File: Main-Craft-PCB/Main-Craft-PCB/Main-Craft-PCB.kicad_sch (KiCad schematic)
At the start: 216 parts, among them J1 Conn_01x10, J1 UART_1, J10 S500_2, J11 S500_3, J12 S500_4, J13 SOL_1, J14 SOL_2, J15 RELAY_1, J16 RELAY_2, J17 RELAY_3, J18 RELAY_3, J19 SOL_3, J2 UART_2, J20 SOL_4, J21 PWR_IN, J23 BAT_IN, J24 VESC_1, J25 VESC_2, J26 VESC_3, J27 VESC_4, J3 UART_3, J4 UART_4, J5 LEDS, J6 LEDS, J7 LEDS, J8 LEDS, J9 S500_1, Q1 TIP120, Q10 S9013, Q11 S9013, Q12 S9013, Q13 S9013, Q14 S9013, Q16 S9013, Q2 TIP120, Q25 IRFR9014PBF, Q3 TIP120, Q4 TIP120, Q5 S9013, Q6 S9013, Q7 S9013, Q8 S9013, Q9 S9013, U10 BFU590GX, U10 ZLDO1117G50TA, U2 NUCLEO144-F429ZI, U2 Pi Pico, U3 ESP8266, U4 LM358DR2G, U4 SN74LV4052, U5 74HC14, U5 LM358DR2G, U8 74HC14, U9 ZSR330GTA

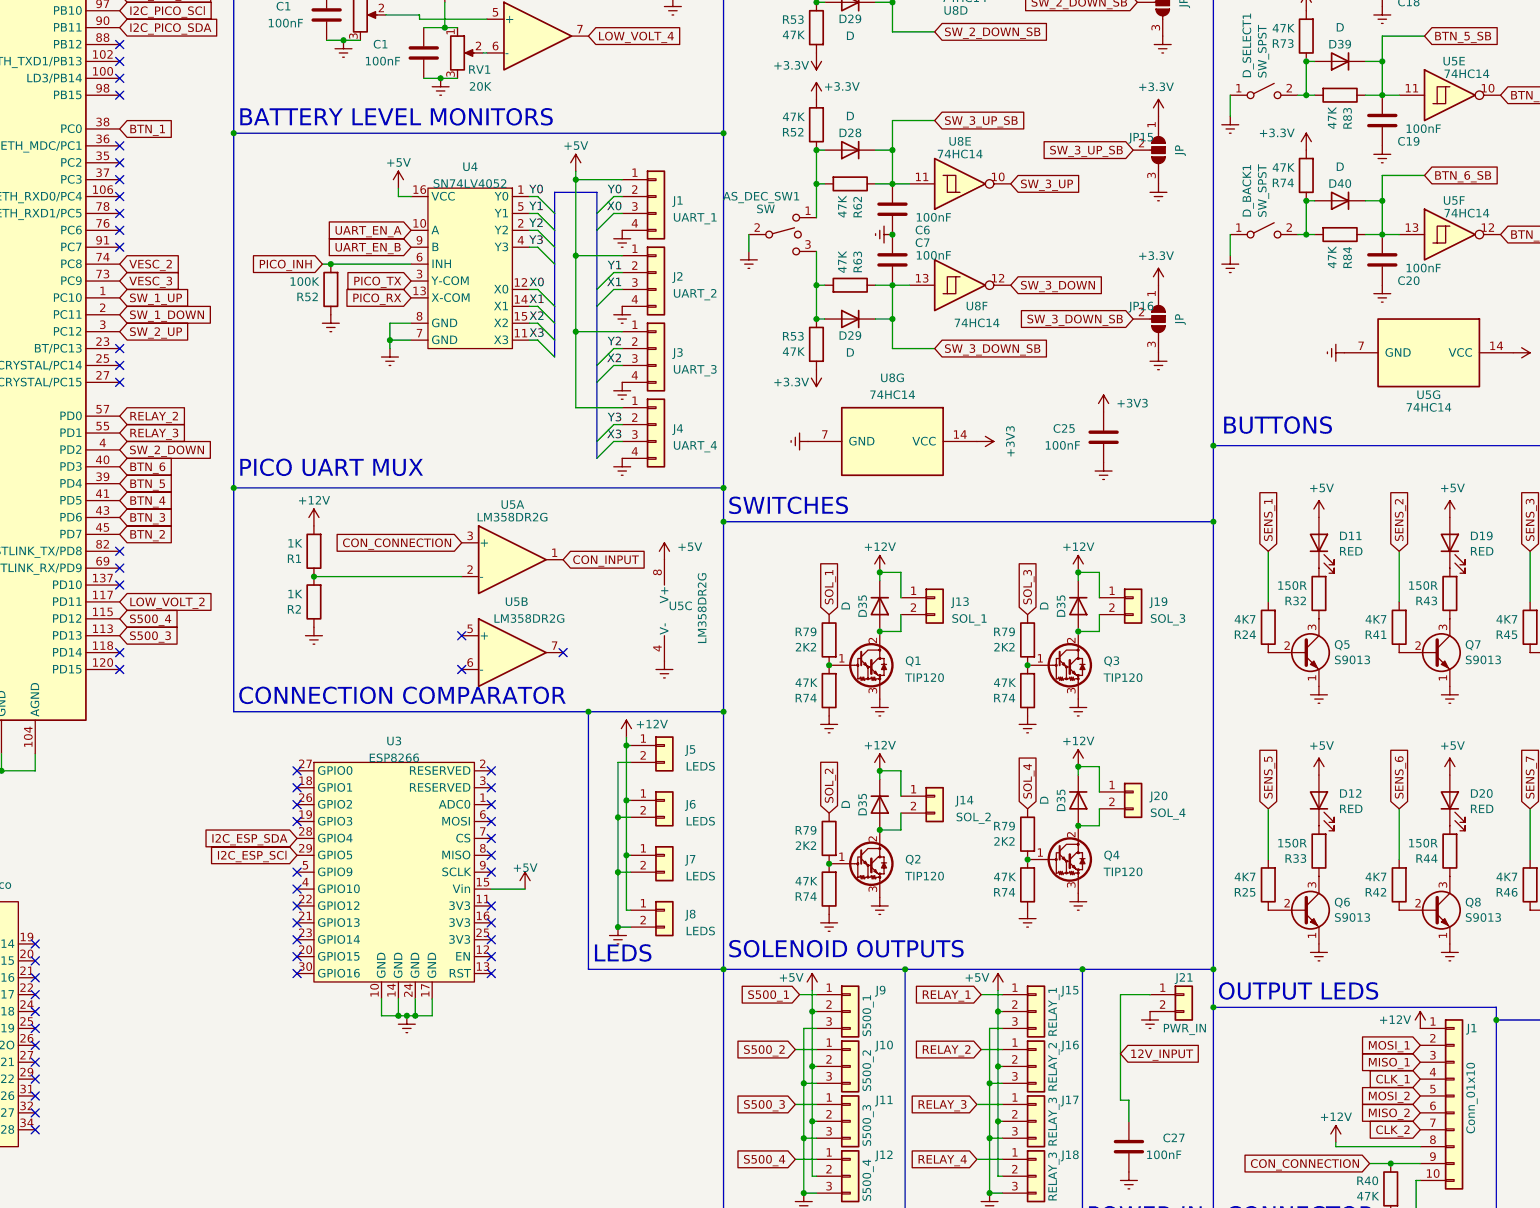
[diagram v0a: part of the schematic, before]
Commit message: Finish PCB ready for checking
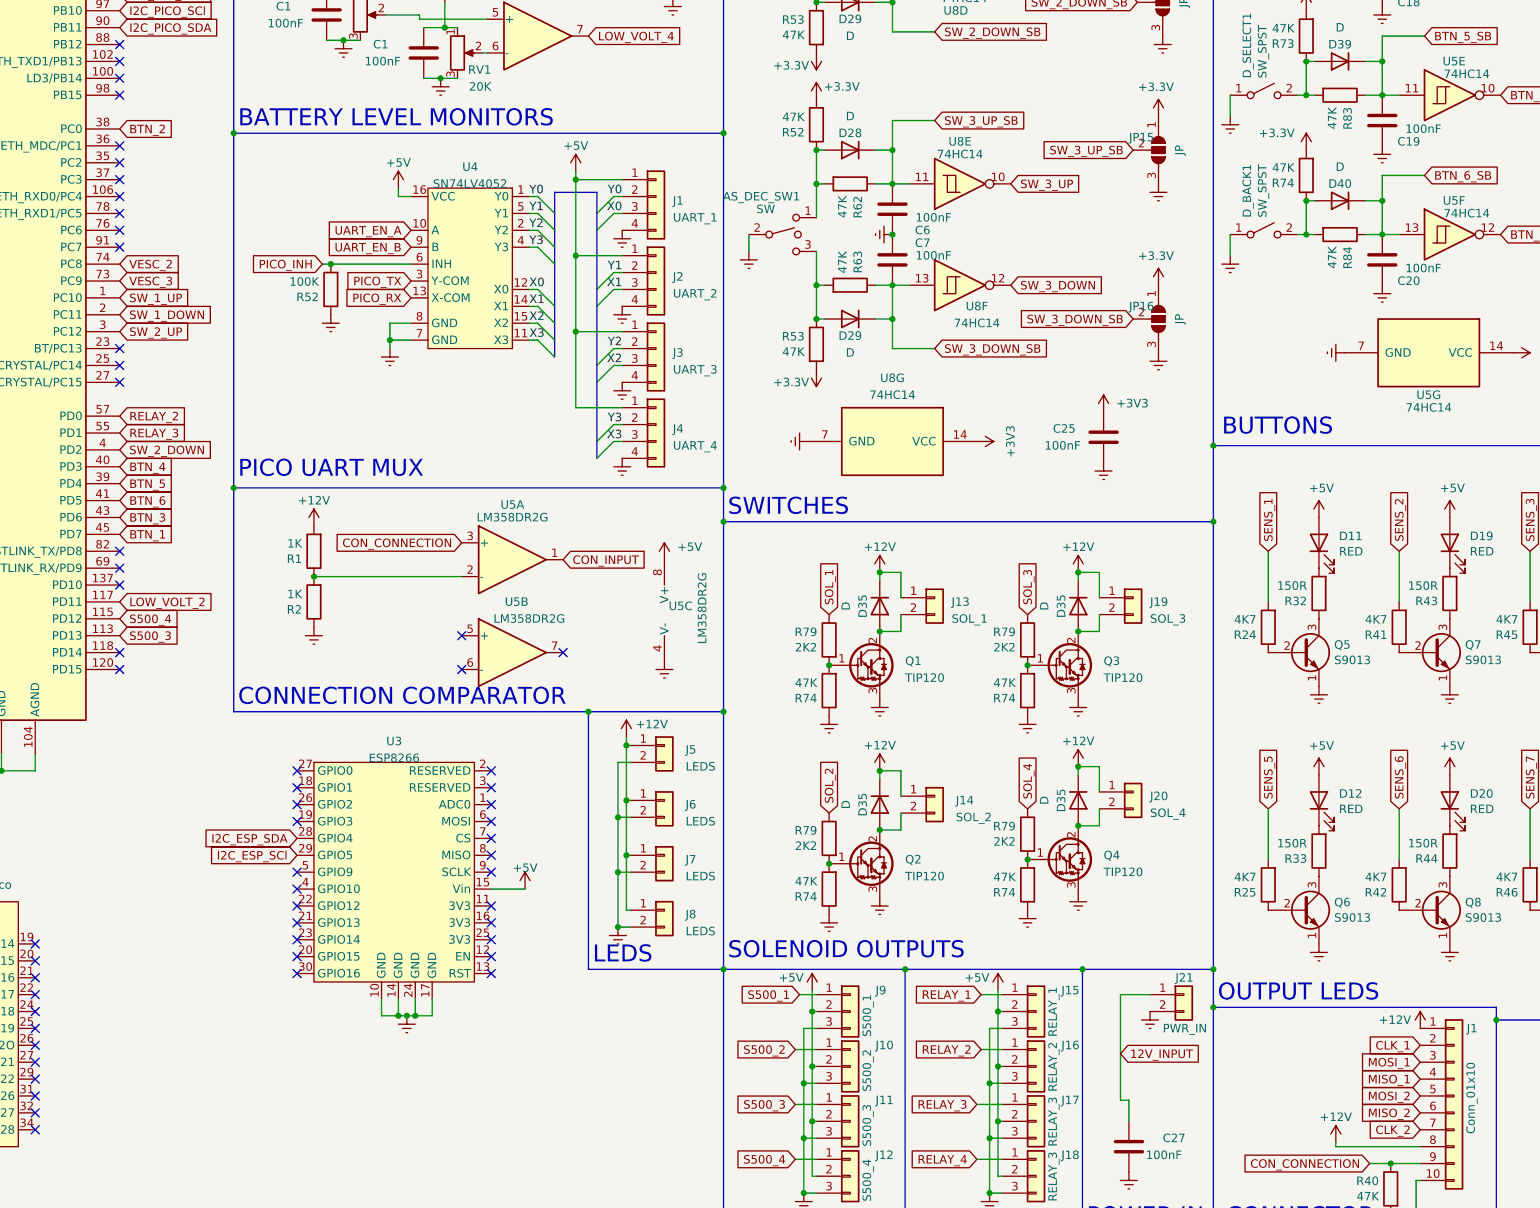
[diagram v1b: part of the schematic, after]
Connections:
- net BTN_1: now also U2.45 (PD7); no longer U2.38 (PC0)
- net BTN_2: now also U2.38 (PC0); no longer U2.45 (PD7)
- net BTN_4: now also U2.40 (PD3); no longer U2.41 (PD5)
- net BTN_6: now also U2.41 (PD5); no longer U2.40 (PD3)
- net CLK_1: now also J1.2 (Pin_2); no longer J1.4 (Pin_4)
- net MISO_1: now also J1.4 (Pin_4); no longer J1.3 (Pin_3)
- net MOSI_1: now also J1.3 (Pin_3); no longer J1.2 (Pin_2)

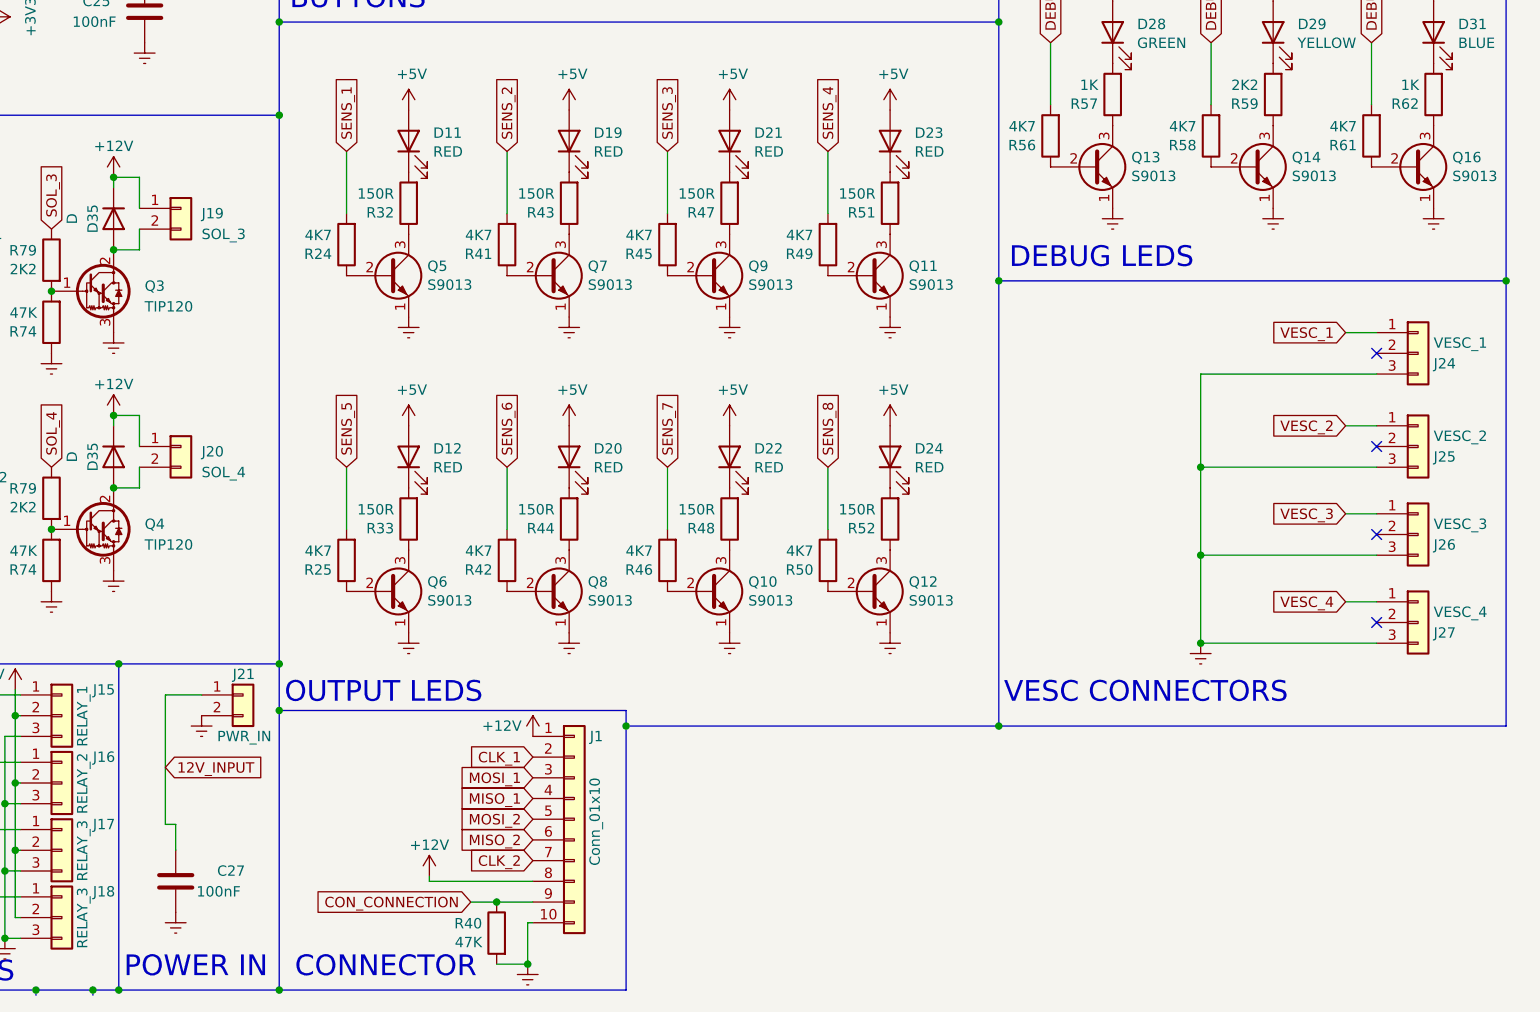
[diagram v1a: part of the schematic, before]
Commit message: Add final touches to PCB
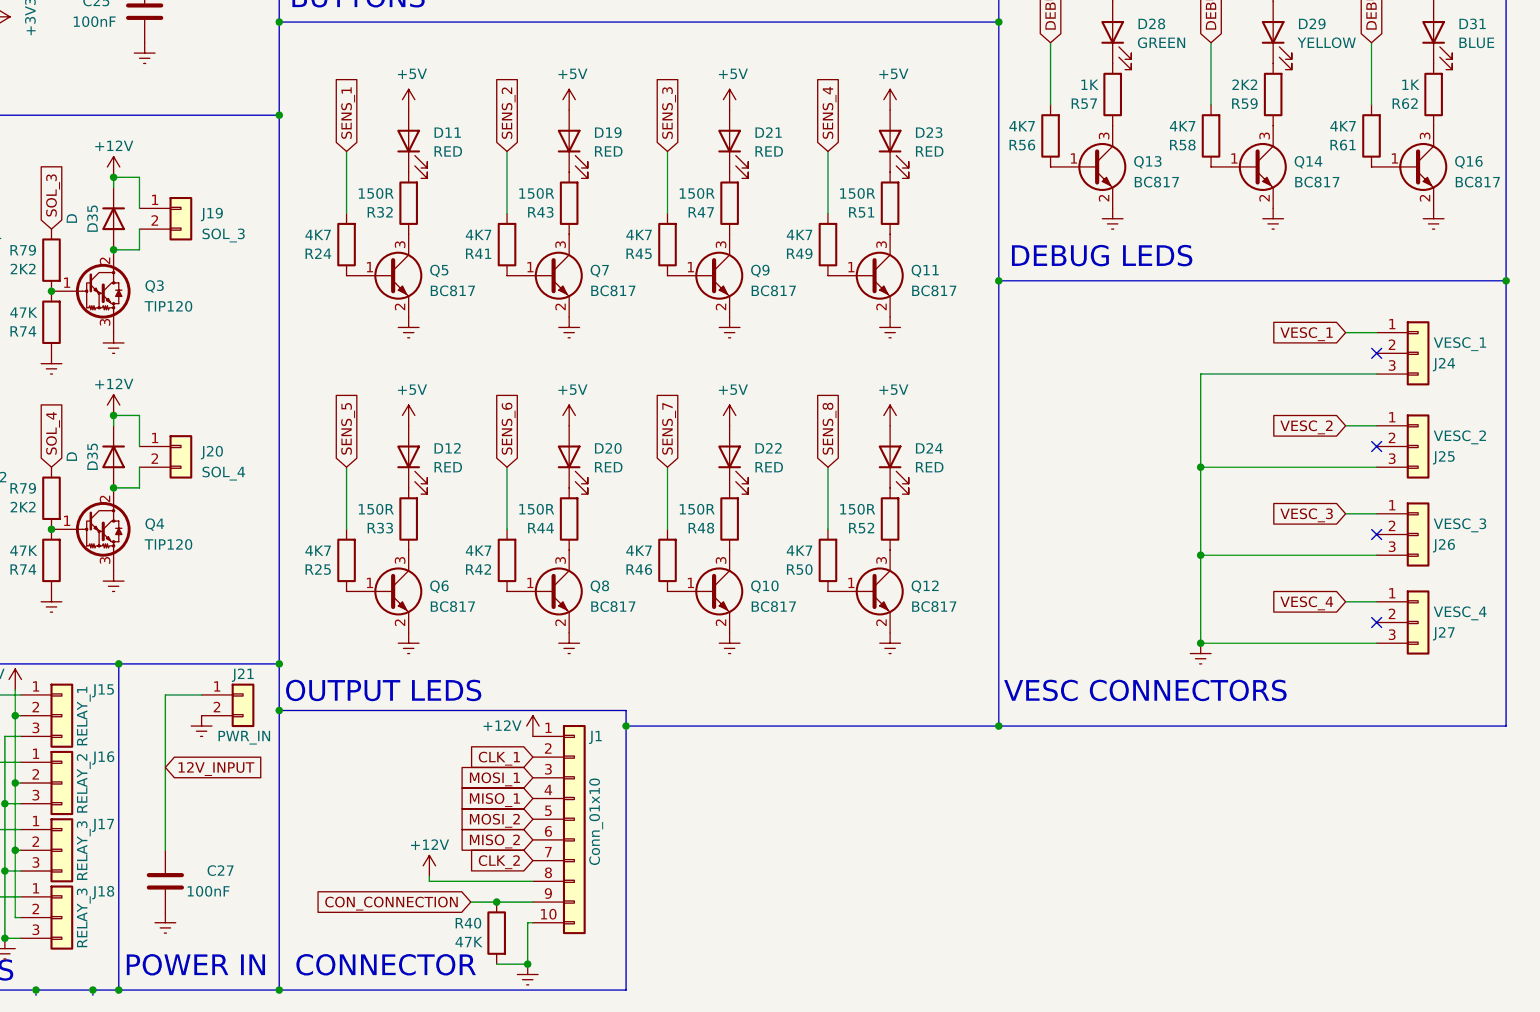
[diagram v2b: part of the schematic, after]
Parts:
- removed Q10, Q11, Q12, Q13, Q14, Q16, Q5, Q6, Q7, Q8, Q9: S9013, Package_TO_SOT_SMD:SOT-23, symbol Transistor_BJT:2N2219
- added Q10, Q11, Q12, Q13, Q14, Q16, Q5, Q6, Q7, Q8, Q9: BC817, Package_TO_SOT_SMD:SOT-23, symbol Transistor_BJT:BC817
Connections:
- net Earth: now also Q10.2 (E), Q11.2 (E), Q12.2 (E), Q13.2 (E), Q14.2 (E), Q16.2 (E), Q5.2 (E), Q6.2 (E), Q7.2 (E), Q8.2 (E), Q9.2 (E)
- net at R44.1: now also Q8.3 (C)
- net at R50.1: now also Q12.1 (B)
- net at R52.1: now also Q12.3 (C)
- net at R41.1: now also Q7.1 (B)
- net at R24.1: now also Q5.1 (B)
- net at R58.1: now also Q14.1 (B)
- net at R59.1: now also Q14.3 (C)
- net at R56.1: now also Q13.1 (B)
- net at R33.1: now also Q6.3 (C)
- net at R45.1: now also Q9.1 (B)
- net at R47.1: now also Q9.3 (C)
- net at R48.1: now also Q10.3 (C)
- net at R49.1: now also Q11.1 (B)
- net at R46.1: now also Q10.1 (B)
- net at R61.1: now also Q16.1 (B)
- net at R62.1: now also Q16.3 (C)
- net at R51.1: now also Q11.3 (C)
- net at R43.1: now also Q7.3 (C)
- net at R32.1: now also Q5.3 (C)
- net at R25.1: now also Q6.1 (B)
- net at R57.1: now also Q13.3 (C)
- net at R42.1: now also Q8.1 (B)
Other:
- moved on the sheet: C27
